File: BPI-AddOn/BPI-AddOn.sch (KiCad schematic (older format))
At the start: 18 parts, among them J1 RJ45, J2 RJ45, J3 RJ45, P1 DIN10, P10 CONN_01X03, P11 CONN_01X05, P12 CONN_01X05, P13 CONN_01X08, P2 DIN10, P3 DIN10, P4 DIN10, P5 DIN10, P6 DIN10, P7 DIN7, P8 DIN7, P9 CONN_01X03

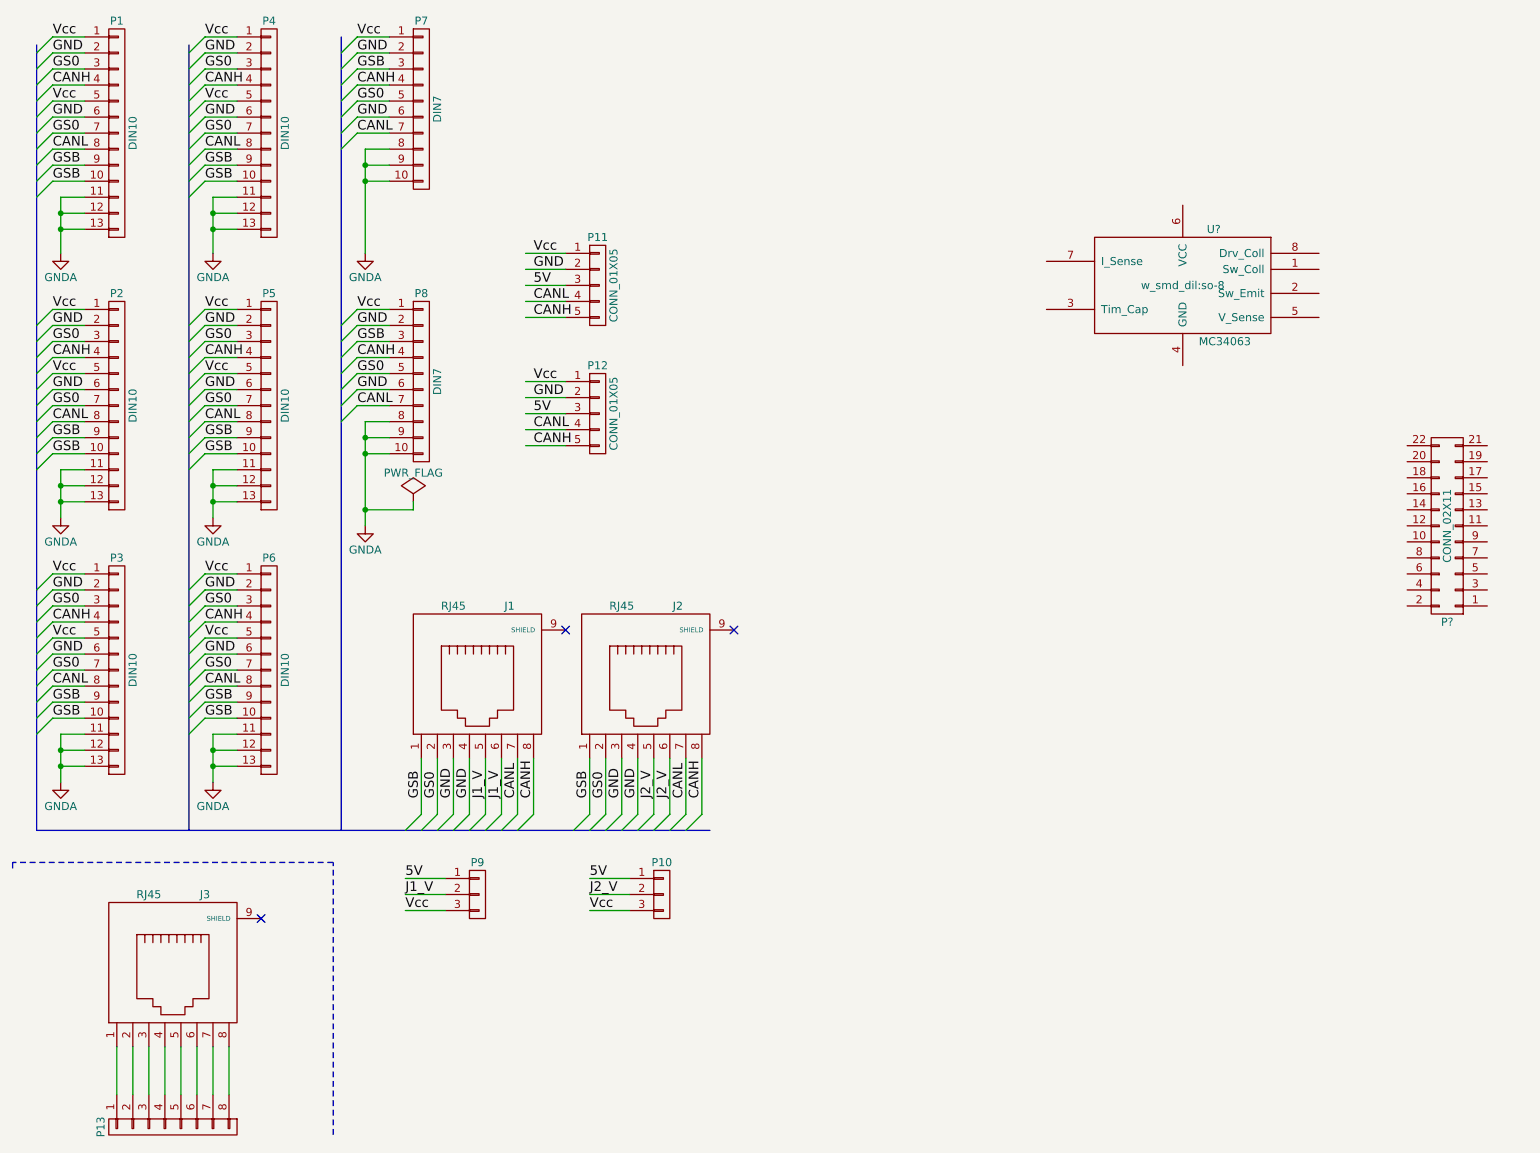
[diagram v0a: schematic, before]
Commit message: wip
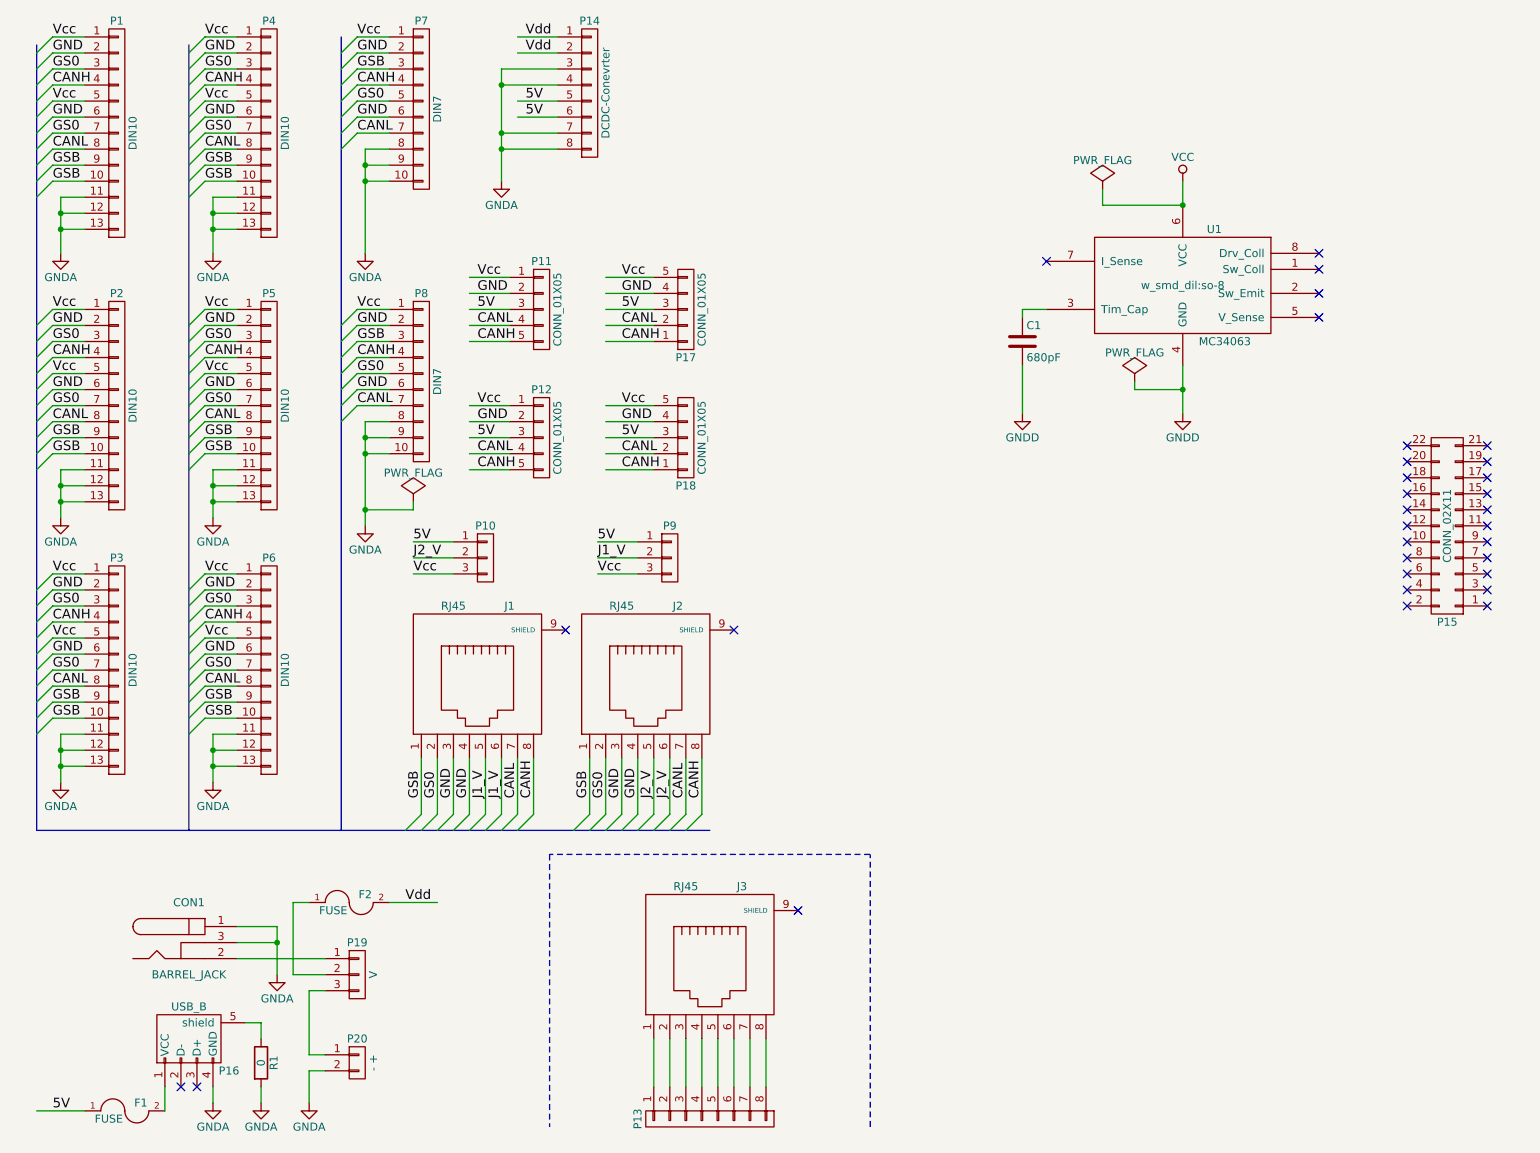
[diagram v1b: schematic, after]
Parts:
- added C1: 680pF, w_capacitors:cnp_3mm_disc, symbol C
- added CON1: BARREL_JACK, w_conn_misc:dc_socket, symbol BARREL_JACK
- added F1, F2: FUSE, Fuse_Holders_and_Fuses:BladeFuse-Mini, symbol FUSE
- added P14: DCDC-Conevrter, 78xx:DCDC, symbol CONN_01X08
- added P16: USB_B, w_conn_pc:conn_usb_B, symbol USB_B
- added P17, P18: CONN_01X05, Pin_Headers:Pin_Header_Straight_1x05, symbol CONN_01X05
- added P19: V, Pin_Headers:Pin_Header_Straight_1x03, symbol CONN_01X03
- added P20: - +, w_conn_pt-1,5:pt_1,5-2-3,5-h, symbol CONN_01X02
- added R1: 0, Resistors_SMD:R_0805_HandSoldering, symbol R
- P15: renamed from P?; footprint (none) -> w_conn_ftsh:ftsh-2211-01-l-dv
- gave numbers to parts that had none: 1
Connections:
- net labels added: GNDD, VCC, Vdd
- wire segments 148 -> 195
- no-connect marks 3 -> 32
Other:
- moved on the sheet: J3, P10, P11, P12, P13, P9

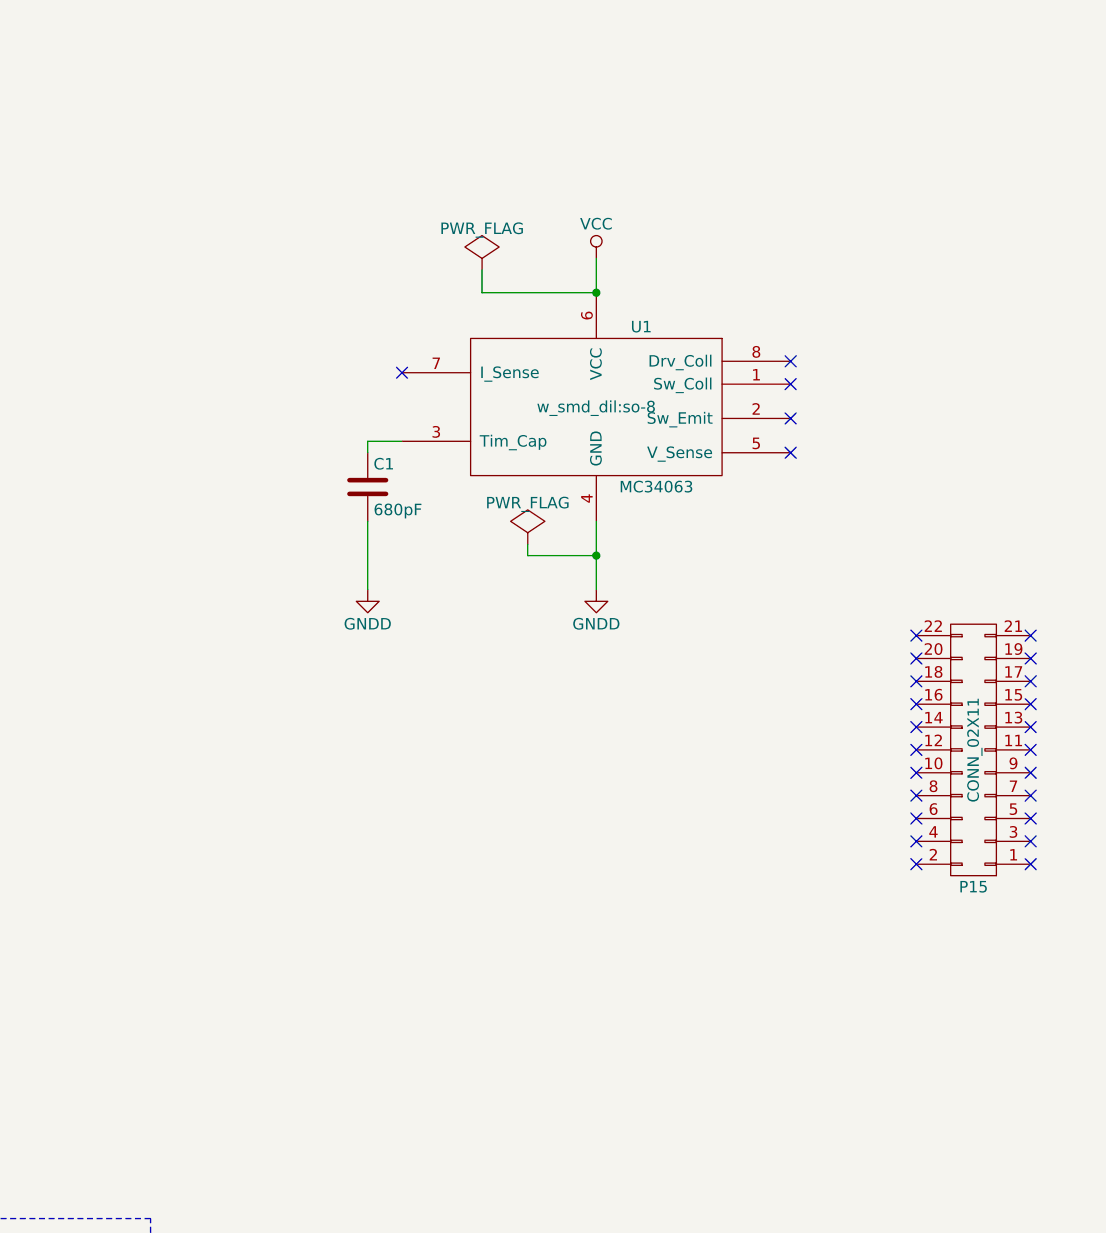
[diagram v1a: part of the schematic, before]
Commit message: working on stepup
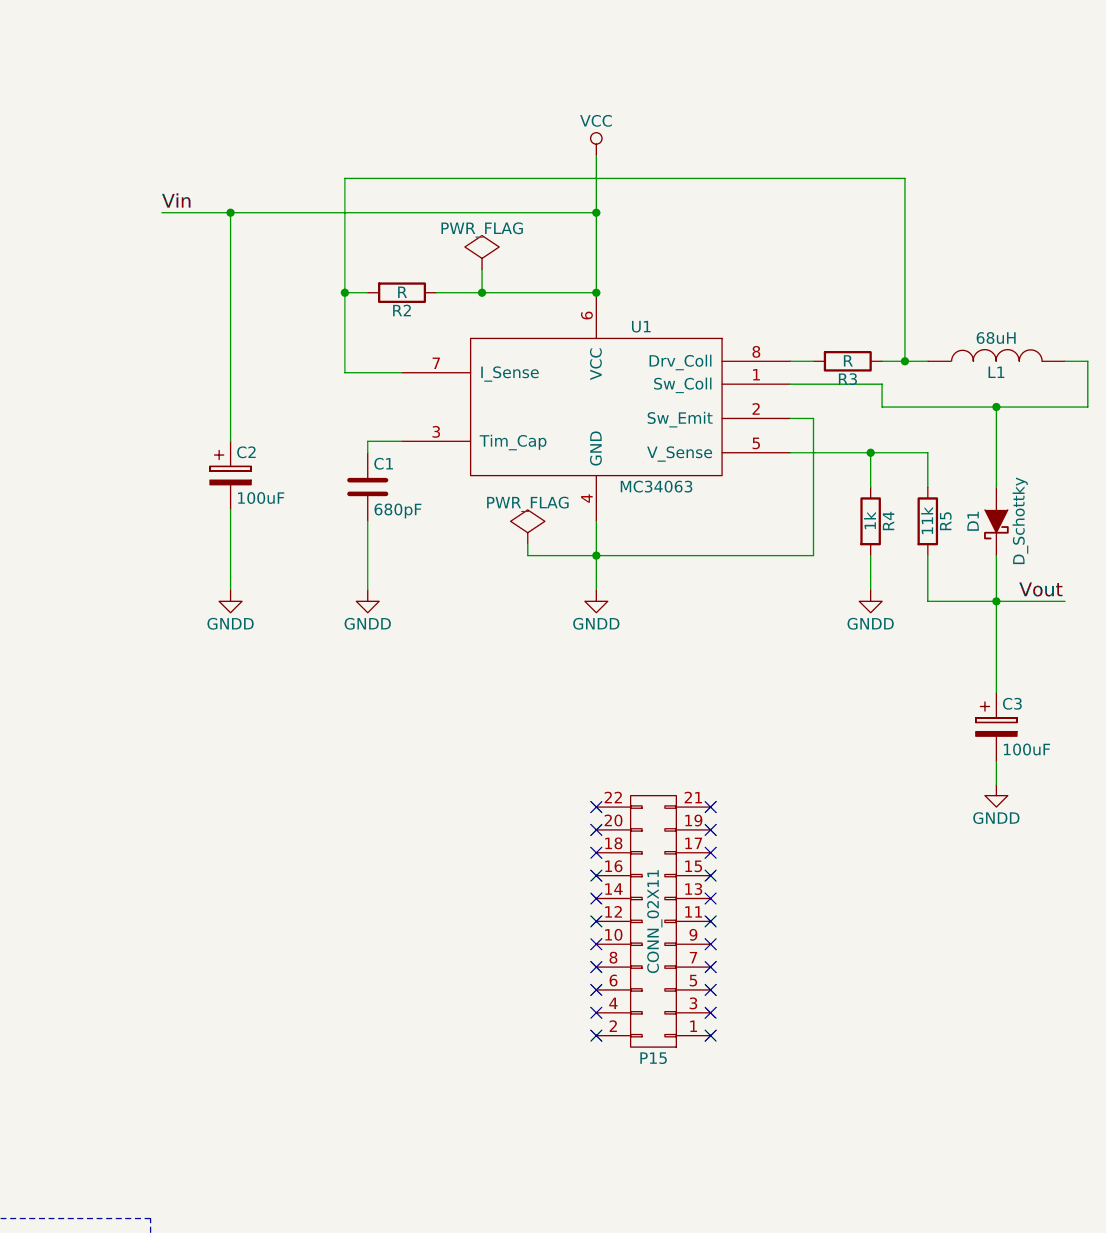
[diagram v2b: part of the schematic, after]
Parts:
- added C2, C3: 100uF, w_capacitors:CP_5x11mm, symbol CP
- added D1: D_Schottky, Diodes_ThroughHole:Diode_DO-35_SOD27_Horizontal_RM10, symbol D_Schottky
- added L1: 68uH, Choke_Radial_ThroughHole:Choke_Radial_27mm_2,8mm-Drills_CD_Bobin_Type_No1410311, symbol INDUCTOR
- added R2, R3: R, w_pth_resistors:RC03, symbol R
- added R4: 1k, w_pth_resistors:RC03, symbol R
- added R5: 11k, w_pth_resistors:RC03, symbol R
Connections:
- net labels added: Vin, Vout
- wire segments 195 -> 221
- no-connect marks 32 -> 27
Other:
- moved on the sheet: P15
